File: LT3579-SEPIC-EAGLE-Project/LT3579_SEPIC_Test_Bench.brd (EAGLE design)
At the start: 300 x 300 mm, 121 parts

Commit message: new files
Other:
- board size 300 x 300 mm -> 178.5 x 182.4 mm
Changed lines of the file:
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@@
 <board>
 <plain>
-<wire x1="0" y1="-100" x2="300" y2="-100" width="0" layer="20"/>
-<wire x1="300" y1="-100" x2="300" y2="200" width="0" layer="20"/>
-<wire x1="300" y1="200" x2="0" y2="200" width="0" layer="20"/>
-<wire x1="0" y1="200" x2="0" y2="-100" width="0" layer="20"/>
+<wire x1="-0.4" y1="-60.45" x2="177.95" y2="-60.45" width="0" layer="20"/>
+<wire x1="177.95" y1="-60.45" x2="178.05" y2="121.9" width="0" layer="20"/>
+<wire x1="178.05" y1="121.9" x2="-0.3" y2="121.9" width="0" layer="20"/>
+<wire x1="-0.3" y1="121.9" x2="-0.4" y2="-60.45" width="0" layer="20"/>
 </plain>
 <attributes>

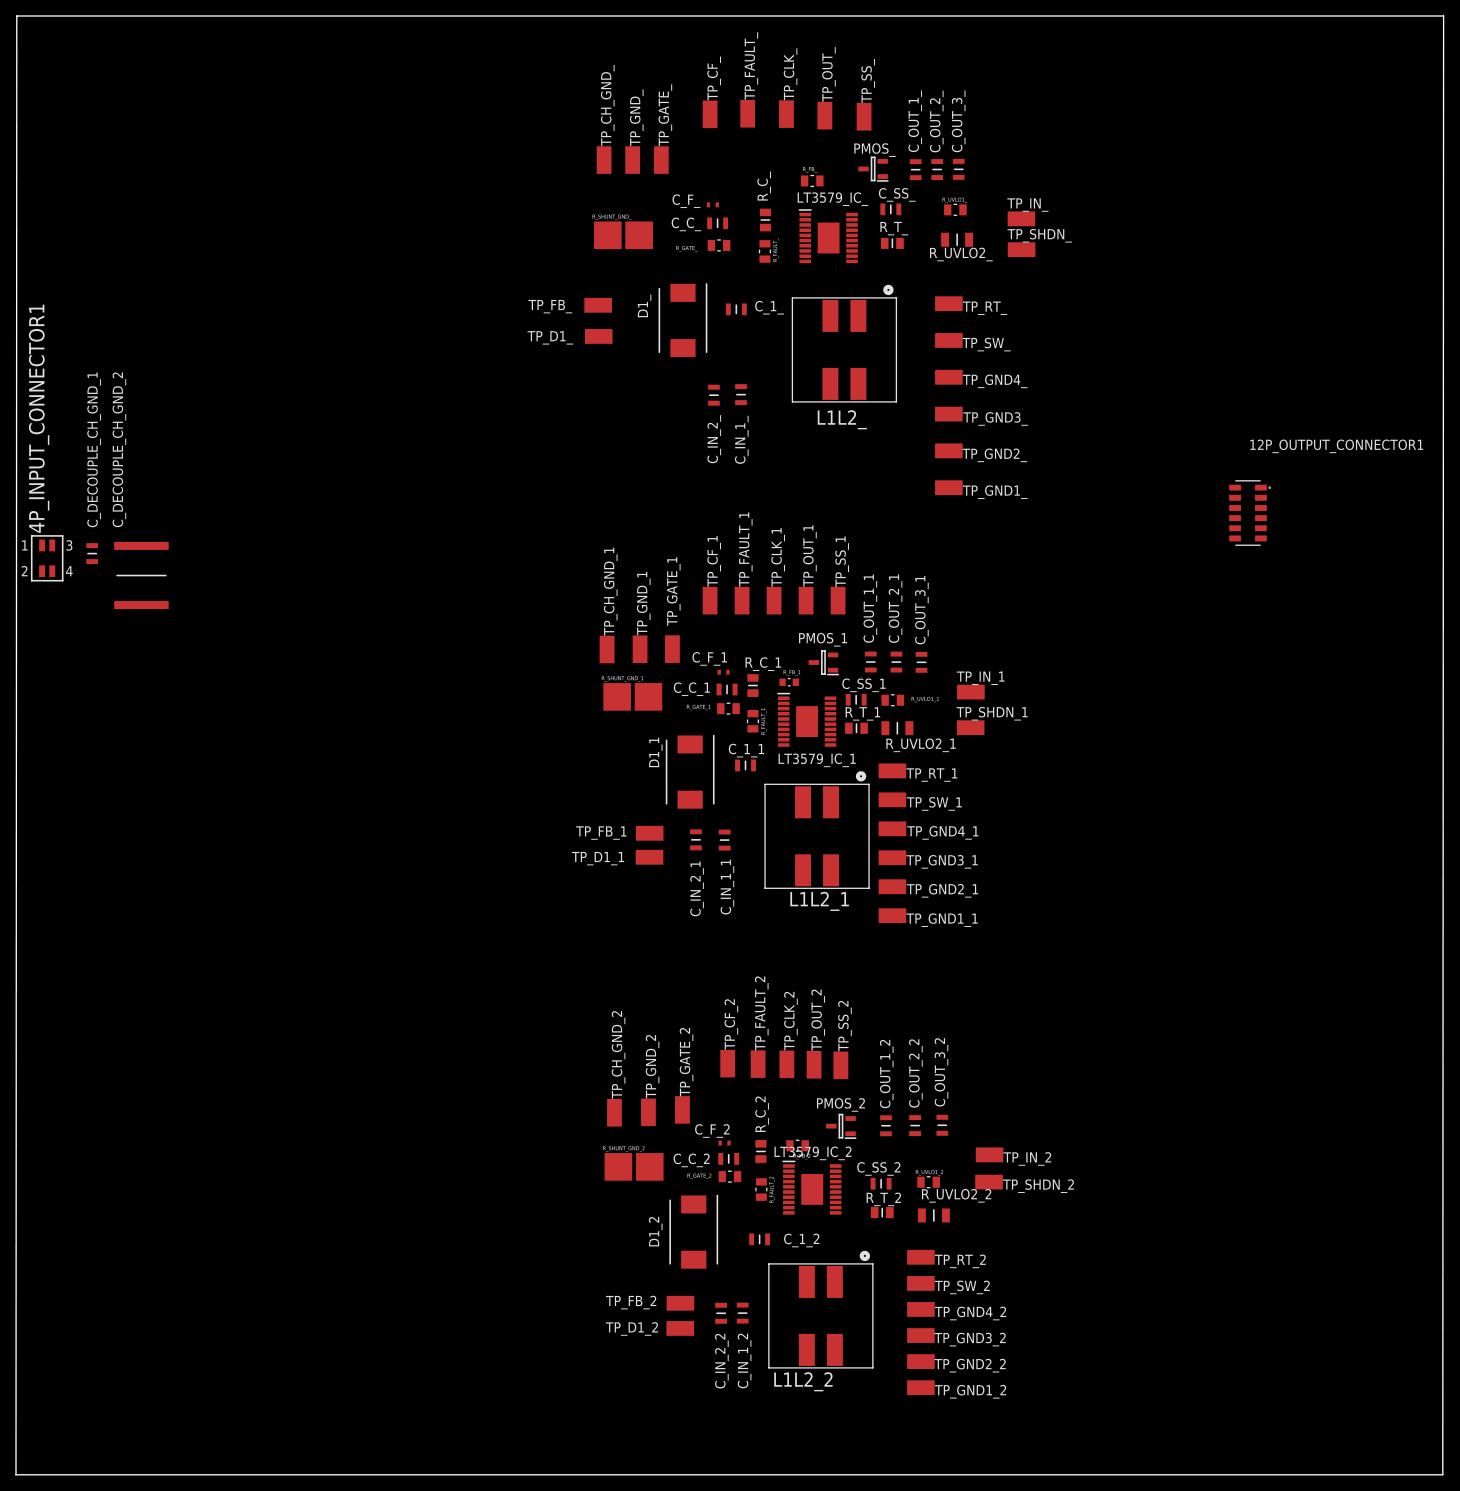
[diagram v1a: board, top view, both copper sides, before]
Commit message: Removed and replaced files
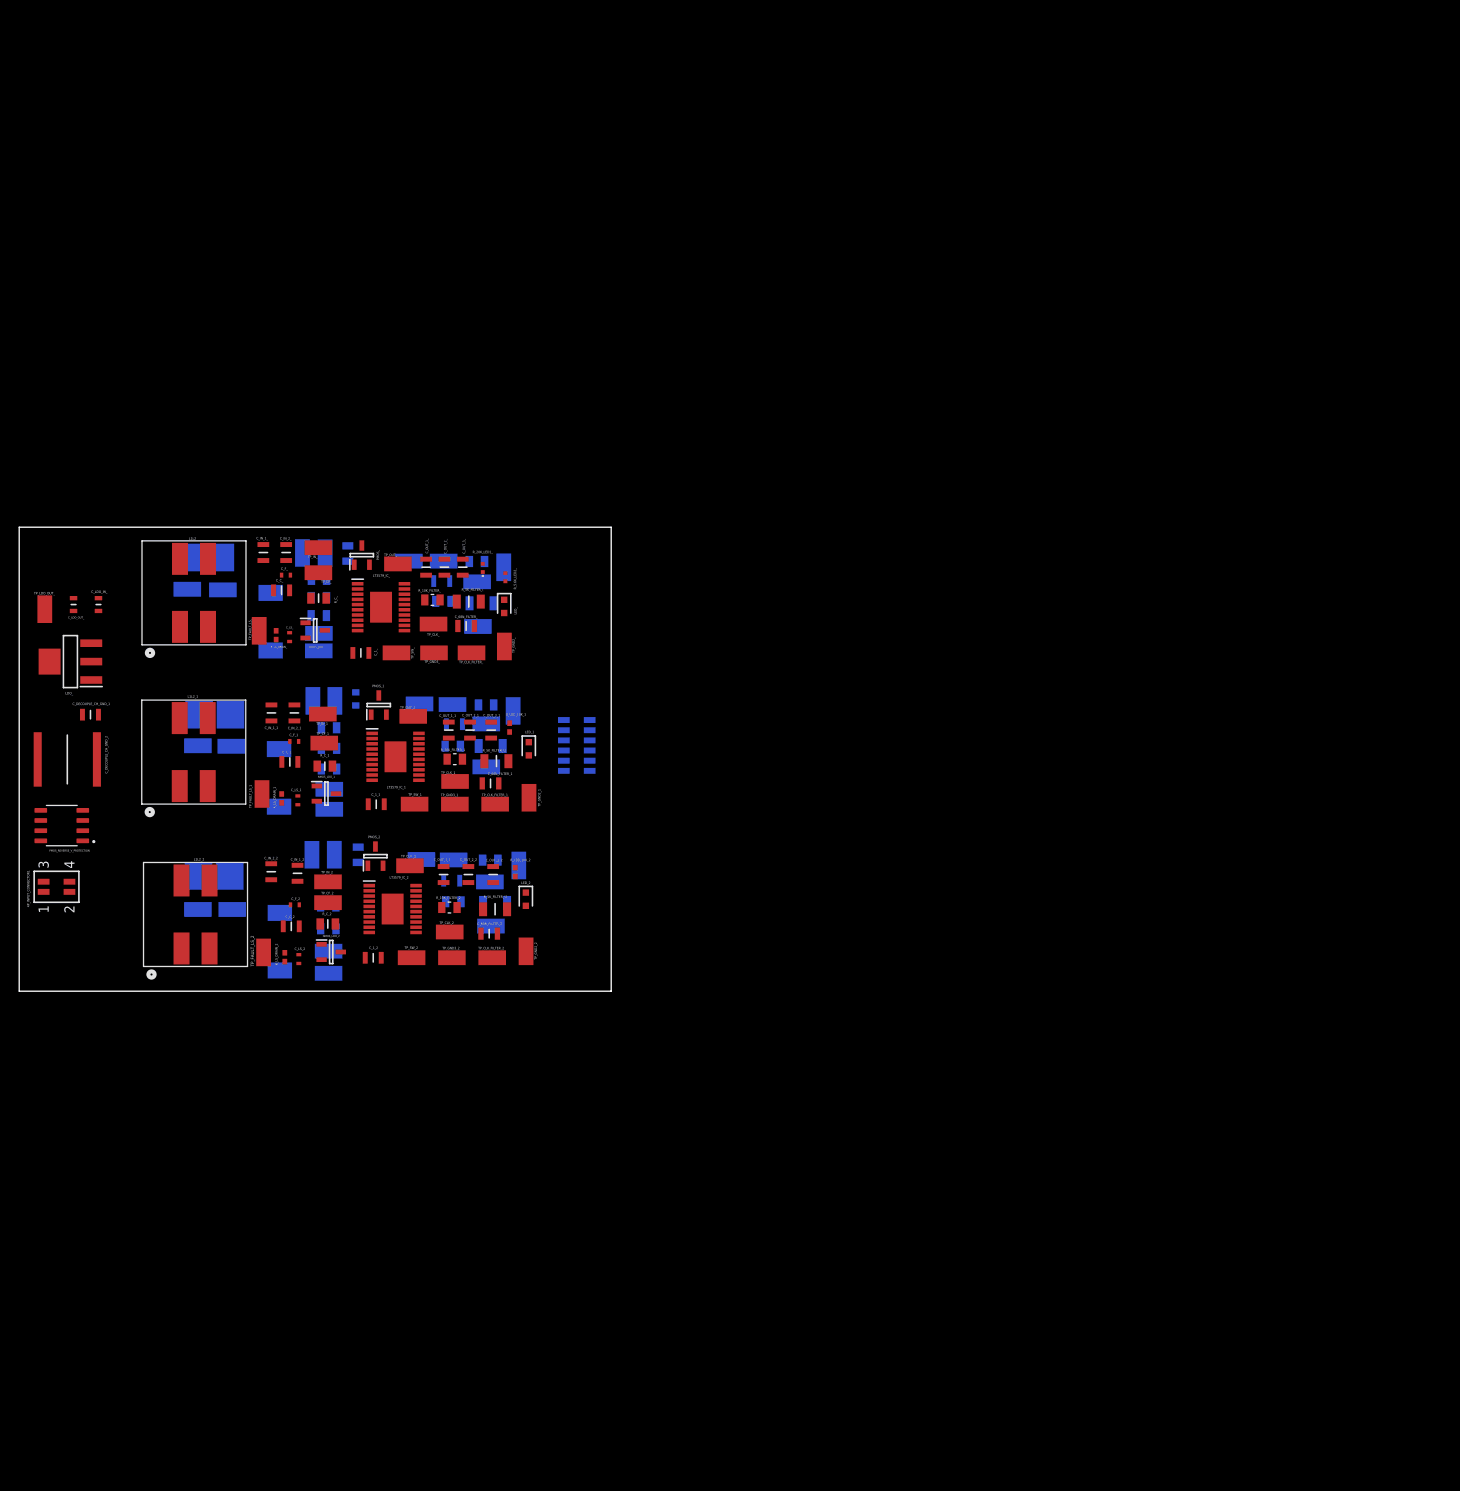
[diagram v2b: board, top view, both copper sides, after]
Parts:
- added C_68N_FILTER_, C_68N_FILTER_1, C_68N_FILTER_2: CEU4J2X7R1H683K125AE, SamacSys_Parts:CAPC2013X150N
- added C_LDO_IN_: CGA3E1X7R1V105K080AC, SamacSys_Parts:CAPC1608X90N
- added C_LDO_OUT_: JMK107BB7475KA-T, SamacSys_Parts:CAPC1608X90N
- added C_LS_, C_LS_1, C_LS_2: CGA2B2C0G1H102J050BE, SamacSys_Parts:CAPC1005X55N
- added LDO_: LDL1117S33R, SamacSys_Parts:SOT230P700X180-4N
- added LED_, LED_1, LED_2: APTD1608LCGCK, SamacSys_Parts:APT1608CGCK
- added NMOS_LDO_, NMOS_LDO_1, NMOS_LDO_2: RSR025N03HZGTL, SamacSys_Parts:SOT95P280X100-3N
- added PMOS_REVERSE_V_PROTECTION: DMP3015LSSQ-13, DMP3015LSSQ-13:SOIC127P600X170-8N
- added R_10K_FILTER_, R_10K_FILTER_1, R_10K_FILTER_2: AC0805DR-0710KL, AC0805DR-0710KL:RESC2012X60N
- added R_20K_LED1_: ERJ-2RKF2002X, SamacSys_Parts:ERJ2R_(0402)
- added R_5.6K_LED2_: ERA-2ARB562X, SamacSys_Parts:ERA2AED122X
- added R_5K_FILTER_\, R_5K_FILTER_\1, R_5K_FILTER_\2: RT1206BRD075KL, SamacSys_Parts:RESC3116X65N
- added R_LED_10K_1, R_LED_10K_2, R_LS_DRAIN_, R_LS_DRAIN_1, R_LS_DRAIN_2: MCS0402MD1002DE000, SamacSys_Parts:RESC1005X37N
- added R_LS_GATE_, R_LS_GATE_1, R_LS_GATE_2: AT0805FRE07100KL, AT0805FRE07100KL:RESC2012X60N
- added TP_CLK_FILTER_, TP_CLK_FILTER_1, TP_CLK_FILTER_2, TP_FAULT_LS_, TP_FAULT_LS_1, TP_FAULT_LS_2, TP_LDO_OUT_: S1751-46R, S1751-46R:S1751-46R_
- D1_, D1_1, D1_2: value MBRS360T3G -> MBRS330T3G; device SamacSys_Parts:DIOM8059X261N -> SamacSys_Parts:DIOM7958X256N
- R_GATE_, R_GATE_1, R_GATE_2: value AC0805DR-0710KL -> AC0805FR-0710KL; device AC0805DR-0710KL:RESC2012X60N -> SamacSys_Parts:RESC2012X60N
- moved TP_IN_ 97.0 mm to (37.4, 55.4)
- moved L1L2_2 92.9 mm to (22.0, 9.59), turned to 180 degrees
- moved TP_GND1_2 90.9 mm to (50.3, 16.5), flipped to the bottom, turned to 180 degrees
- moved TP_IN_2 89.5 mm to (38.6, 13.7)
- moved 12P_OUTPUT_CONNECTOR1 88.8 mm to (69.7, 30.7), flipped to the bottom
- moved L1L2_ 86.8 mm to (21.9, 49.8), turned to 180 degrees
- moved TP_FAULT_ 84.2 mm to (37.5, 44.7), flipped to the bottom, turned to 0 degrees
- moved TP_SHDN_ 82.7 mm to (57.3, 45.6), flipped to the bottom
- moved TP_IN_1 81.0 mm to (38.0, 34.6)
- moved R_UVLO1_ 80.6 mm to (53.0, 48.7), flipped to the bottom, turned to 180 degrees
- moved PMOS_ 80.1 mm to (42.8, 54.5), turned to 90 degrees
- moved C_OUT_3_ 79.5 mm to (55.4, 53.0)
- moved TP_SW_ 79.3 mm to (47.2, 42.3)
- moved C_OUT_2_ 79.2 mm to (53.1, 53.0)
- moved C_OUT_1_ 78.8 mm to (50.9, 53.0)
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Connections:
- new net CLK_FILTER_OUT_: 12P_OUTPUT_CONNECTOR1.6, C_68N_FILTER_.1, R_10K_FILTER_.2, R_5K_FILTER_\.1, TP_CLK_FILTER_.1
- new net CLK_FILTER_OUT_1: 12P_OUTPUT_CONNECTOR1.4, C_68N_FILTER_1.1, R_10K_FILTER_1.2, R_5K_FILTER_\1.1, TP_CLK_FILTER_1.1
- new net CLK_FILTER_OUT_2: 12P_OUTPUT_CONNECTOR1.2, C_68N_FILTER_2.1, R_10K_FILTER_2.2, R_5K_FILTER_\2.1, TP_CLK_FILTER_2.1
- new net FAULT_LS_OUT_: 12P_OUTPUT_CONNECTOR1.5, C_LS_.1, NMOS_LDO_.3, R_LS_DRAIN_.1, TP_FAULT_LS_.1
- new net FAULT_LS_OUT_1: 12P_OUTPUT_CONNECTOR1.3, C_LS_1.1, NMOS_LDO_1.3, R_LS_DRAIN_1.1, TP_FAULT_LS_1.1
- new net FAULT_LS_OUT_2: 12P_OUTPUT_CONNECTOR1.1, C_LS_2.1, NMOS_LDO_2.3, R_LS_DRAIN_2.1, TP_FAULT_LS_2.1
- new net LDO_OUT_: C_LDO_OUT_.1, LDO_.2, LDO_.4, R_LS_DRAIN_.2, R_LS_DRAIN_1.2, R_LS_DRAIN_2.2, TP_LDO_OUT_.1
- new net N$10: NMOS_LDO_1.1, R_LS_GATE_1.2
- new net N$11: LED_1.1, R_LED_10K_1.2
- new net N$12: R_20K_LED1_.1, R_5.6K_LED2_.1
- new net N$14: NMOS_LDO_2.1, R_LS_GATE_2.2
- new net N$15: LED_.1, R_5.6K_LED2_.2
- new net N$16: LED_2.1, R_LED_10K_2.2
- new net N$8: NMOS_LDO_.1, R_LS_GATE_.2
- new net VIN_CONNECTOR: 4P_INPUT_CONNECTOR1.1, 4P_INPUT_CONNECTOR1.3, PMOS_REVERSE_V_PROTECTION.5, PMOS_REVERSE_V_PROTECTION.6, PMOS_REVERSE_V_PROTECTION.7, PMOS_REVERSE_V_PROTECTION.8
- net 0: now also C_68N_FILTER_.2, C_68N_FILTER_1.2, C_68N_FILTER_2.2, C_LDO_IN_.2, C_LDO_OUT_.2, C_LS_.2, C_LS_1.2, C_LS_2.2, LED_.2, LED_1.2, LED_2.2, NMOS_LDO_.2, NMOS_LDO_1.2, NMOS_LDO_2.2, PMOS_REVERSE_V_PROTECTION.4, R_5K_FILTER_\.2, R_5K_FILTER_\1.2, R_5K_FILTER_\2.2
- net CLK_: now also R_10K_FILTER_.1; no longer 12P_OUTPUT_CONNECTOR1.6
- net CLK_1: now also R_10K_FILTER_1.1; no longer 12P_OUTPUT_CONNECTOR1.4
- net CLK_2: now also R_10K_FILTER_2.1; no longer 12P_OUTPUT_CONNECTOR1.2
- net FAULT_: now also R_LS_GATE_.1; no longer 12P_OUTPUT_CONNECTOR1.5
- net FAULT_1: now also R_LS_GATE_1.1; no longer 12P_OUTPUT_CONNECTOR1.3
- net FAULT_2: now also R_LS_GATE_2.1; no longer 12P_OUTPUT_CONNECTOR1.1
- net GND: now also LDO_.1
- net VIN: now also C_LDO_IN_.1, LDO_.3, PMOS_REVERSE_V_PROTECTION.1, PMOS_REVERSE_V_PROTECTION.2, PMOS_REVERSE_V_PROTECTION.3; no longer 4P_INPUT_CONNECTOR1.1, 4P_INPUT_CONNECTOR1.3
- net VOUT_: now also R_20K_LED1_.2
- net VOUT_1: now also R_LED_10K_1.1
- net VOUT_2: now also R_LED_10K_2.1
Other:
- board size 178.5 x 182.4 mm -> 74 x 58 mm
